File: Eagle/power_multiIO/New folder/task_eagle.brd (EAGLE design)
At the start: 85 x 123.9 mm, 100 parts, among them IC2 ATMEGA640-16AI, IC3 74ACT125D, IC7 FT232RL, IC8 MAX485, K1 G5LE, K2 G5LE, K3 G5LE, K6 G5LE, U1 TC1262-33VDB, U2 Tyco 5-6605758-1, U3 ENC28J60-SSOP, Y2 25MHz

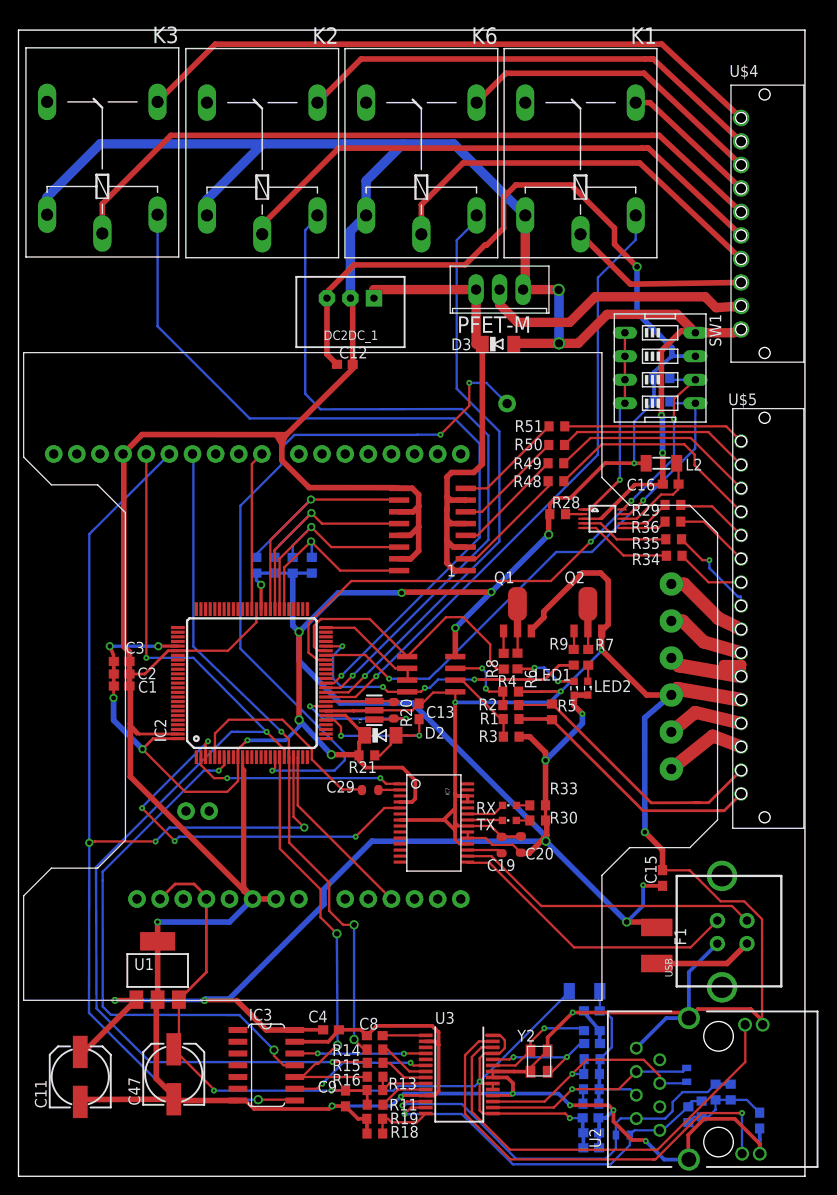
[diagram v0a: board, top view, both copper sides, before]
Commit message: rfid and power_multiIO
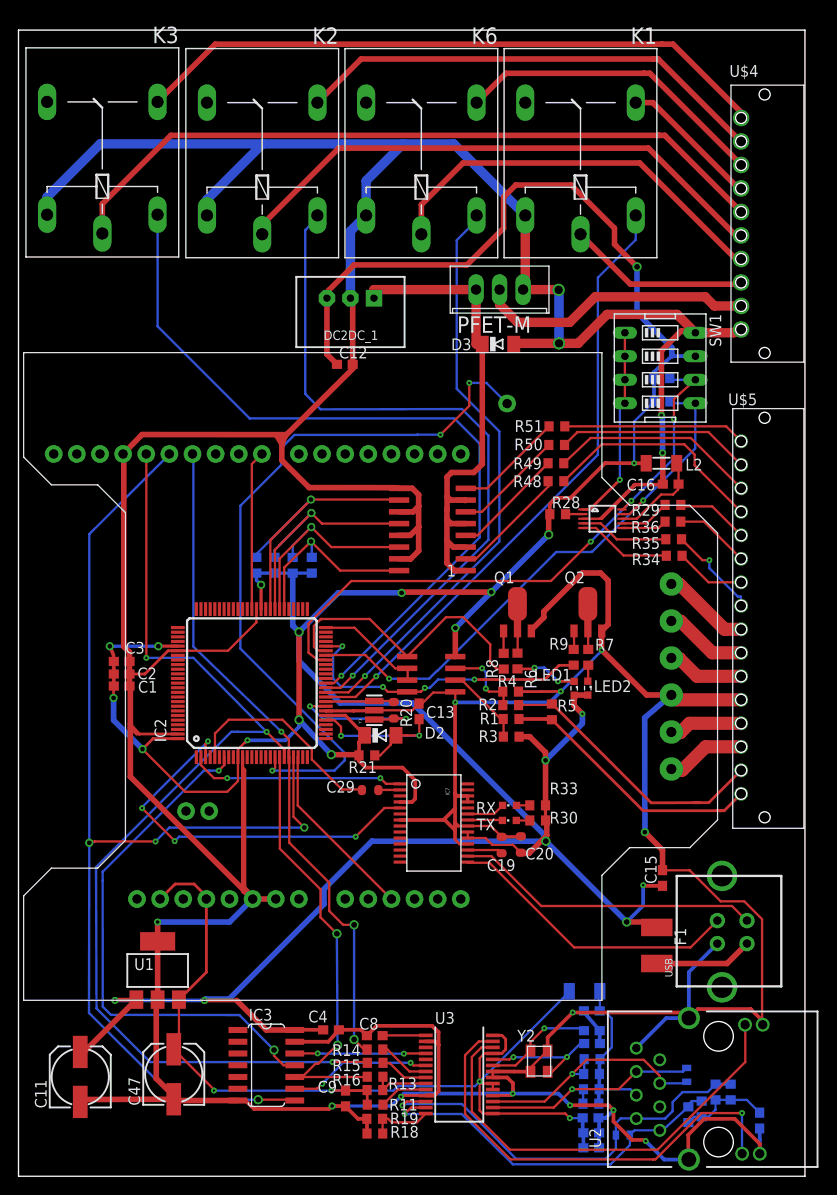
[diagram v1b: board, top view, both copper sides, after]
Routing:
- net VMOT: track 11.6 -> 8.37 mm
- net 12V_IN: track 30.8 -> 30.1 mm
